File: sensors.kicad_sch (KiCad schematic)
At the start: 43 parts

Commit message: started routing
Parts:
- R? (x4): footprint Resistor_SMD:R_0603_1608Metric -> Resistor_SMD:R_0402_1005Metric
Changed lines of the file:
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@@
       (effects (font (size 1.27 1.27)) (justify left))
     )
-    (property "Footprint" "Resistor_SMD:R_0603_1608Metric" (at 125.222 104.14 90)
+    (property "Footprint" "Resistor_SMD:R_0402_1005Metric" (at 125.222 104.14 90)
       (effects (font (size 1.27 1.27)) hide)
     )
@@
       (effects (font (size 1.27 1.27)) (justify left))
     )
-    (property "Footprint" "Resistor_SMD:R_0603_1608Metric" (at 250.952 156.21 90)
+    (property "Footprint" "Resistor_SMD:R_0402_1005Metric" (at 250.952 156.21 90)
       (effects (font (size 1.27 1.27)) hide)
     )
@@
       (effects (font (size 1.27 1.27)) (justify left))
     )
-    (property "Footprint" "Resistor_SMD:R_0603_1608Metric" (at 31.242 102.87 90)
+    (property "Footprint" "Resistor_SMD:R_0402_1005Metric" (at 31.242 102.87 90)
       (effects (font (size 1.27 1.27)) hide)
     )
@@
       (effects (font (size 1.27 1.27)) (justify left))
     )
-    (property "Footprint" "Resistor_SMD:R_0603_1608Metric" (at 93.472 172.72 90)
-      (effects (font (size 1.27 1.27)) hide)
-    )
+    (property "Footprint" "Resistor_SMD:R_0402_1005Metric" (at 93.472 172.72 90)
+      (effects (font (size 1.27 1.27)) hide)
+    )

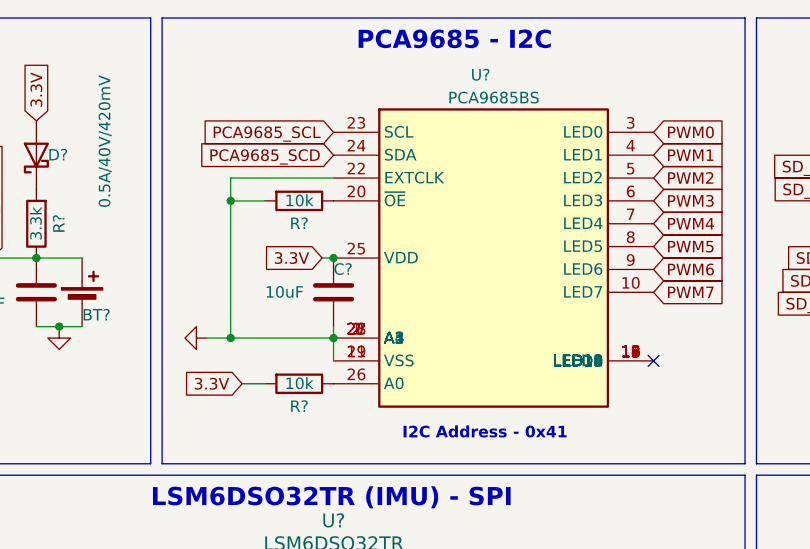
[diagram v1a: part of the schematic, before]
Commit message: more routing
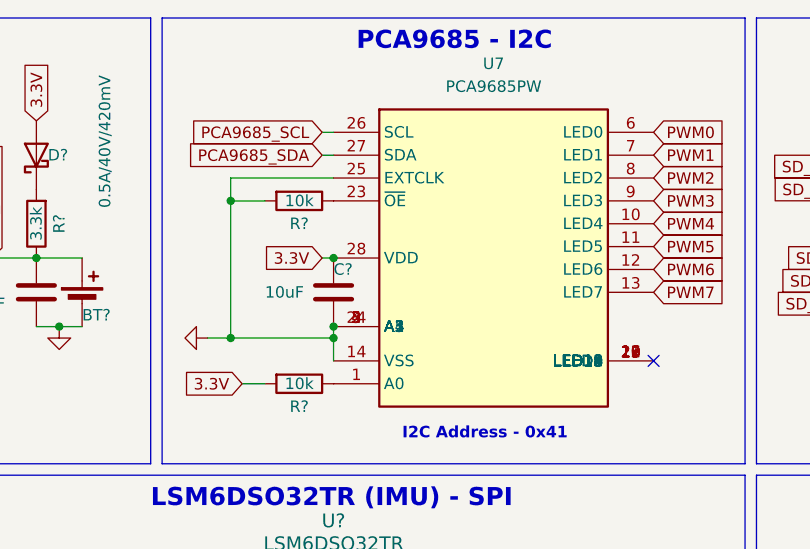
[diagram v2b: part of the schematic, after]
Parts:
- removed U?: PCA9685BS, Package_DFN_QFN:QFN-28-1EP_6x6mm_P0.65mm_EP4.25x4.25mm, symbol Driver_LED:PCA9685BS
- added U7: PCA9685PW, Package_SO:TSSOP-28_4.4x9.7mm_P0.65mm, symbol Driver_LED:PCA9685PW
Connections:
- net 3.3V: now also U7.28 (VDD)
- net GND: now also U7.14 (VSS), U7.2 (A1), U7.24 (A5), U7.25 (EXTCLK), U7.3 (A2), U7.4 (A3), U7.5 (A4)
- net PCA9685_SCL: now also U7.26 (SCL)
- net PWM0: now also U7.6 (LED0)
- net PWM1: now also U7.7 (LED1)
- net PWM2: now also U7.8 (LED2)
- net PWM3: now also U7.9 (LED3)
- net PWM4: now also U7.10 (LED4)
- net PWM5: now also U7.11 (LED5)
- net PWM6: now also U7.12 (LED6)
- net PWM7: now also U7.13 (LED7)
- net at R?.1: now also U7.1 (A0)
- net at R?.1: now also U7.23 (~{OE})
- new net: U7.15 (LED8), U7.16 (LED9), U7.17 (LED10), U7.18 (LED11), U7.19 (LED12), U7.20 (LED13), U7.21 (LED14), U7.22 (LED15)
- new net PCA9685_SDA: U7.27 (SDA)
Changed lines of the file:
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@@
   (junction (at 33.02 166.37) (diameter 0) (color 0 0 0 0)
   )
+  (junction (at 160.02 40.64) (diameter 0) (color 0 0 0 0)
+  )
+  (junction (at 160.02 48.26) (diameter 0) (color 0 0 0 0)
+  )
   (junction (at 218.44 53.34) (diameter 0) (color 0 0 0 0)
   )
@@
   (junction (at 133.35 181.61) (diameter 0) (color 0 0 0 0)
   )
-  (junction (at 160.02 40.64) (diameter 0) (color 0 0 0 0)
-  )
   (no_connect (at 218.44 35.56))
   (no_connect (at 195.58 52.07))
@@
     (stroke (width 0) (type default))
   )
+  (wire (pts (xy 158.75 29.21) (xy 160.02 29.21))
+    (stroke (width 0) (type default))
+  )
   (wire (pts (xy 149.86 54.61) (xy 152.4 54.61))
     (stroke (width 0) (type default))
@@
     (stroke (width 0) (type default))
   )
+  (wire (pts (xy 158.75 26.67) (xy 160.02 26.67))
+    (stroke (width 0) (type default))
+  )
   (wire (pts (xy 133.35 181.61) (xy 133.35 182.88))
     (stroke (width 0) (type default))
@@
     )
   )
-  (global_label "PCA9685_SCD" (shape input) (at 160.02 29.21 180) (fields_autoplaced)
+  (global_label "PCA9685_SDA" (shape input) (at 158.75 29.21 180) (fields_autoplaced)
     (effects (font (size 1.27 1.27)) (justify right))
-    (property "Intersheetrefs" "${INTERSHEET_REFS}" (at 143.8511 29.21 0)
+    (property "Intersheetrefs" "${INTERSHEET_REFS}" (at 142.7625 29.21 0)
       (effects (font (size 1.27 1.27)) (justify right) hide)
     )
@@
     )
   )
-  (global_label "PCA9685_SCL" (shape input) (at 160.02 26.67 180) (fields_autoplaced)
+  (global_label "PCA9685_SCL" (shape input) (at 158.75 26.67 180) (fields_autoplaced)
     (effects (font (size 1.27 1.27)) (justify right))
-    (property "Intersheetrefs" "${INTERSHEET_REFS}" (at 144.093 26.67 0)
+    (property "Intersheetrefs" "${INTERSHEET_REFS}" (at 142.823 26.67 0)
       (effects (font (size 1.27 1.27)) (justify right) hide)
     )
@@
     )
   )
+  (symbol (lib_id "Driver_LED:PCA9685PW") (at 177.8 44.45 0) (unit 1)
+    (in_bom yes) (on_board yes) (dnp no) (fields_autoplaced)
+    (property "Reference" "U7" (at 177.8 19.05 0)
+      (effects (font (size 1.27 1.27)))
+    )
+    (property "Value" "PCA9685PW" (at 177.8 21.59 0)
+      (effects (font (size 1.27 1.27)))
+    )
+    (property "Footprint" "Package_SO:TSSOP-28_4.4x9.7mm_P0.65mm" (at 178.435 69.215 0)
+      (effects (font (size 1.27 1.27)) (justify left) hide)
+    )
+    (property "Datasheet" "http://www.nxp.com/docs/en/data-sheet/PCA9685.pdf" (at 167.64 26.67 0)
+      (effects (font (size 1.27 1.27)) hide)
+    )
+    (pin "1")
+    (pin "10")
+    (pin "11")
+    (pin "12")
+    (pin "13")
+    (pin "14")
+    (pin "15")
+    (pin "16")
+    (pin "17")
+    (pin "18")
+    (pin "19")
+    (pin "2")
+    (pin "20")
+    (pin "21")
+    (pin "22")
+    (pin "23")
+    (pin "24")
+    (pin "25")
+    (pin "26")
+    (pin "27")
+    (pin "28")
+    (pin "3")
+    (pin "4")
+    (pin "5")
+    (pin "6")
+    (pin "7")
+    (pin "8")
+    (pin "9")
+    (instances
+      (project "aether"
+        (path "/e12346fa-509d-4de9-8ab1-dced307292db/b5ec7ecd-943d-4169-981a-c46b6432f873"
+          (reference "U7") (unit 1)
+        )
+      )
+    )
+  )
   (symbol (lib_id "power:GND") (at 218.44 55.88 0) (unit 1)
     (in_bom yes) (on_board yes) (dnp no) (fields_autoplaced)
@@
         )
       )
-    )
-  )
-  (symbol (lib_id "Driver_LED:PCA9685BS") (at 177.8 44.45 0) (unit 1)
-    (in_bom yes) (on_board yes) (dnp no)
-    (property "Reference" "U?" (at 175.26 20.32 0)
-      (effects (font (size 1.27 1.27)) (justify left))
-    )
-    (property "Value" "PCA9685BS" (at 172.72 22.86 0)
-      (effects (font (size 1.27 1.27)) (justify left))
-    )
-    (property "Footprint" "Package_DFN_QFN:QFN-28-1EP_6x6mm_P0.65mm_EP4.25x4.25mm" (at 178.435 69.215 0)
-      (effects (font (size 1.27 1.27)) (justify left) hide)
-    )
-    (property "Datasheet" "http://www.nxp.com/docs/en/data-sheet/PCA9685.pdf" (at 167.64 26.67 0)
-      (effects (font (size 1.27 1.27)) hide)
-    )
-    (pin "1")
-    (pin "10")
-    (pin "11")
-    (pin "12")
-    (pin "13")
-    (pin "14")
-    (pin "15")
-    (pin "16")
-    (pin "17")
-    (pin "18")
-    (pin "19")
-    (pin "2")
-    (pin "20")
-    (pin "21")
-    (pin "22")
-    (pin "23")
-    (pin "24")
-    (pin "25")
-    (pin "26")
-    (pin "27")
-    (pin "28")
-    (pin "29")
-    (pin "3")
-    (pin "4")
-    (pin "5")
-    (pin "6")
-    (pin "7")
-    (pin "8")
-    (pin "9")
-    (instances
-      (project "aether"
-        (path "/e12346fa-509d-4de9-8ab1-dced307292db"
-          (reference "U?") (unit 1)
-        )
-        (path "/e12346fa-509d-4de9-8ab1-dced307292db/b5ec7ecd-943d-4169-981a-c46b6432f873"
-          (reference "U7") (unit 1)
-        )
-      )

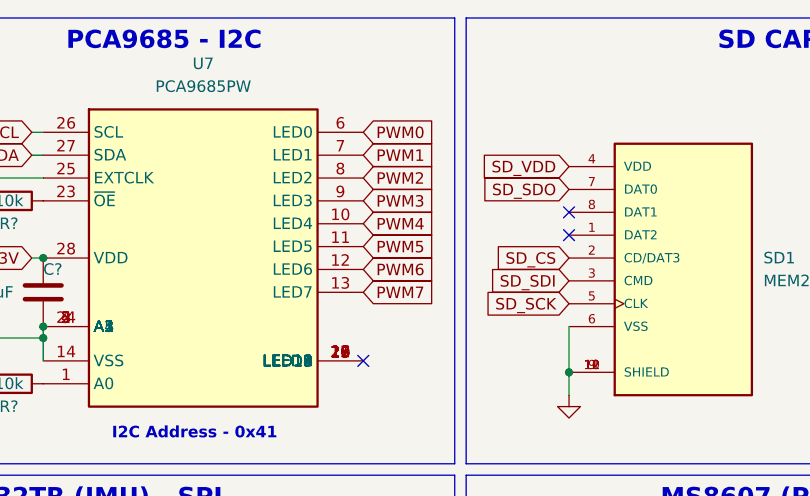
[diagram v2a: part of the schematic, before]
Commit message: significant amount of routing done
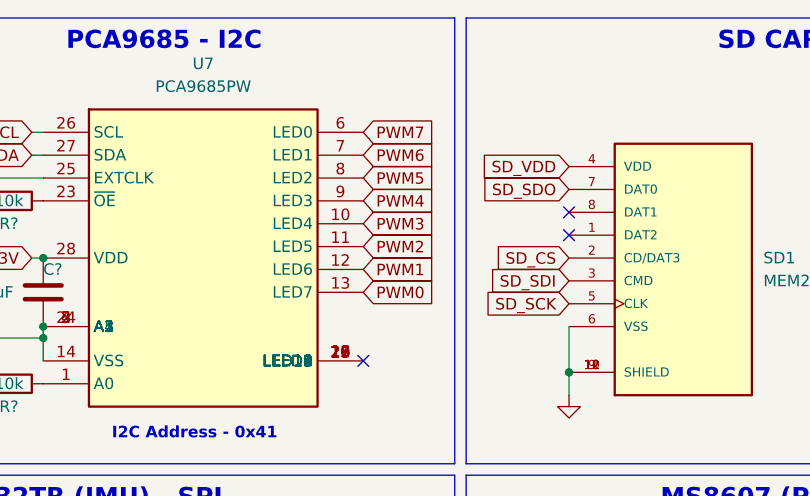
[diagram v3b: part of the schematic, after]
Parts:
- C?: footprint Capacitor_SMD:C_0603_1608Metric -> Capacitor_SMD:C_0402_1005Metric
- D?: footprint LED_SMD:LED_0603_1608Metric -> LED_SMD:LED_0402_1005Metric
- R? (x6): footprint Resistor_SMD:R_0603_1608Metric -> Resistor_SMD:R_0402_1005Metric
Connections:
- net PWM0: now also U7.13 (LED7); no longer U7.6 (LED0)
- net PWM1: now also U7.12 (LED6); no longer U7.7 (LED1)
- net PWM2: now also U7.11 (LED5); no longer U7.8 (LED2)
- net PWM3: now also U7.10 (LED4); no longer U7.9 (LED3)
- net PWM4: now also U7.9 (LED3); no longer U7.10 (LED4)
- net PWM5: now also U7.8 (LED2); no longer U7.11 (LED5)
- net PWM6: now also U7.7 (LED1); no longer U7.12 (LED6)
- net PWM7: now also U7.6 (LED0); no longer U7.13 (LED7)
